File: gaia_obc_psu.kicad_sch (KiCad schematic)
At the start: 49 parts, among them J4 Conn_01x02_Pin, Q1 FS8205A, U10 INA3221, U11 TPS22917DBV, U12 TPS22917DBV, U2 LGS4056H, U3 DW01A, U5 AP2112K-3.3, U8 TPS22917DBV, U9 INA3221

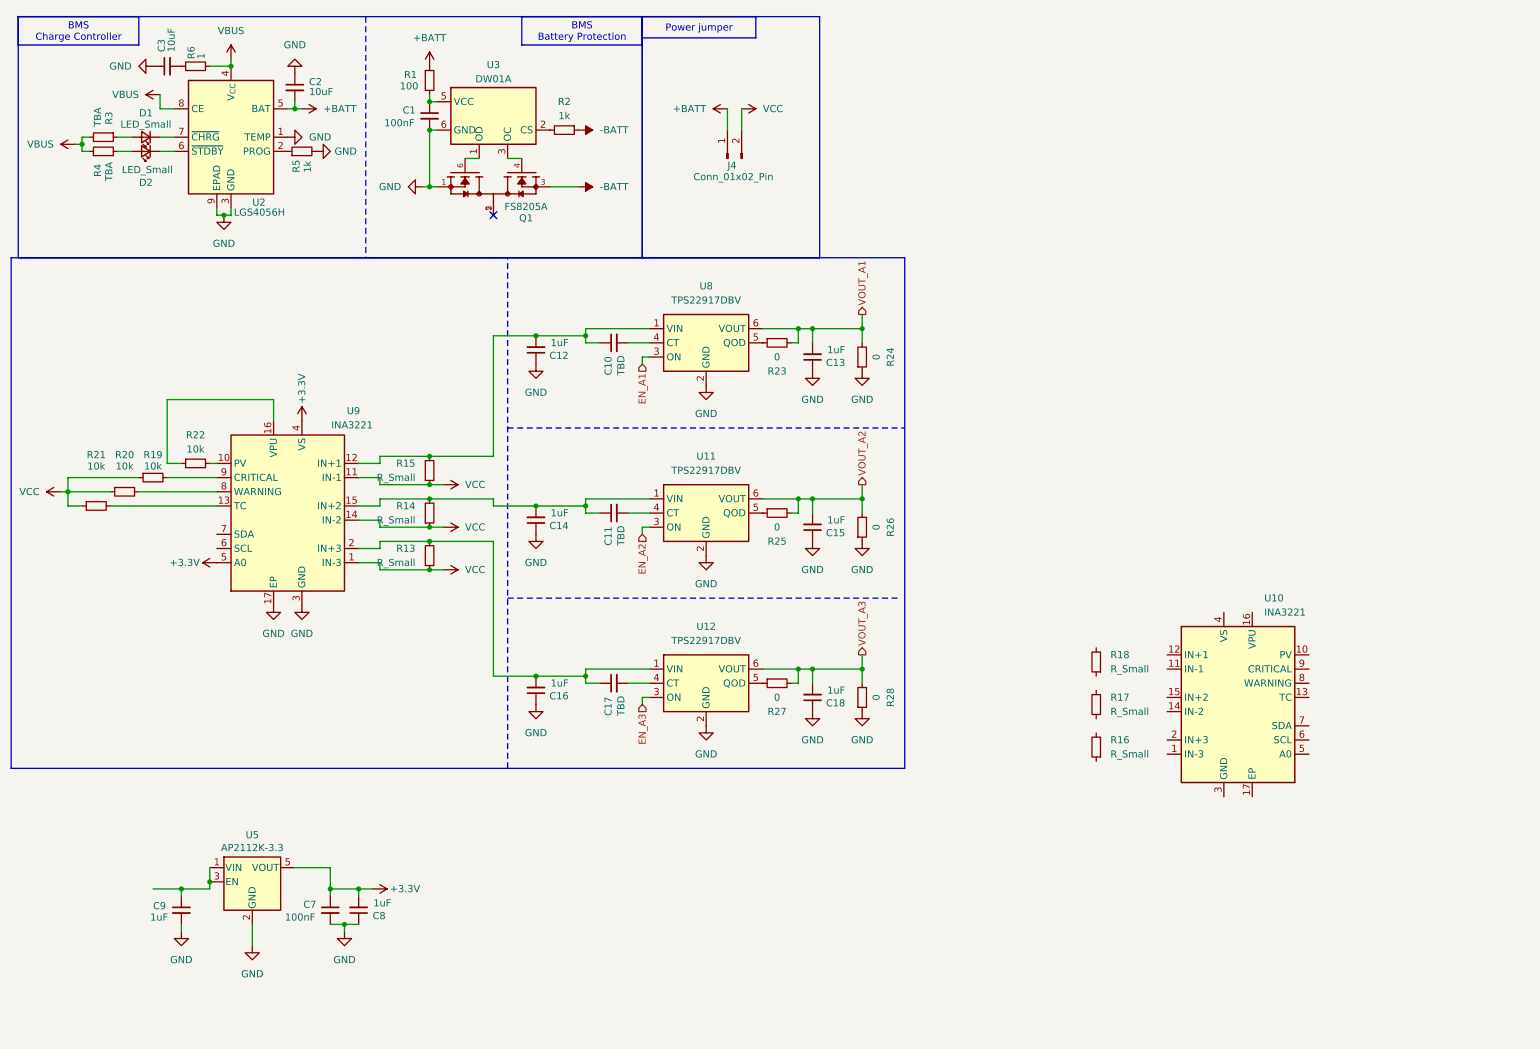
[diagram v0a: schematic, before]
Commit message: finishing psu
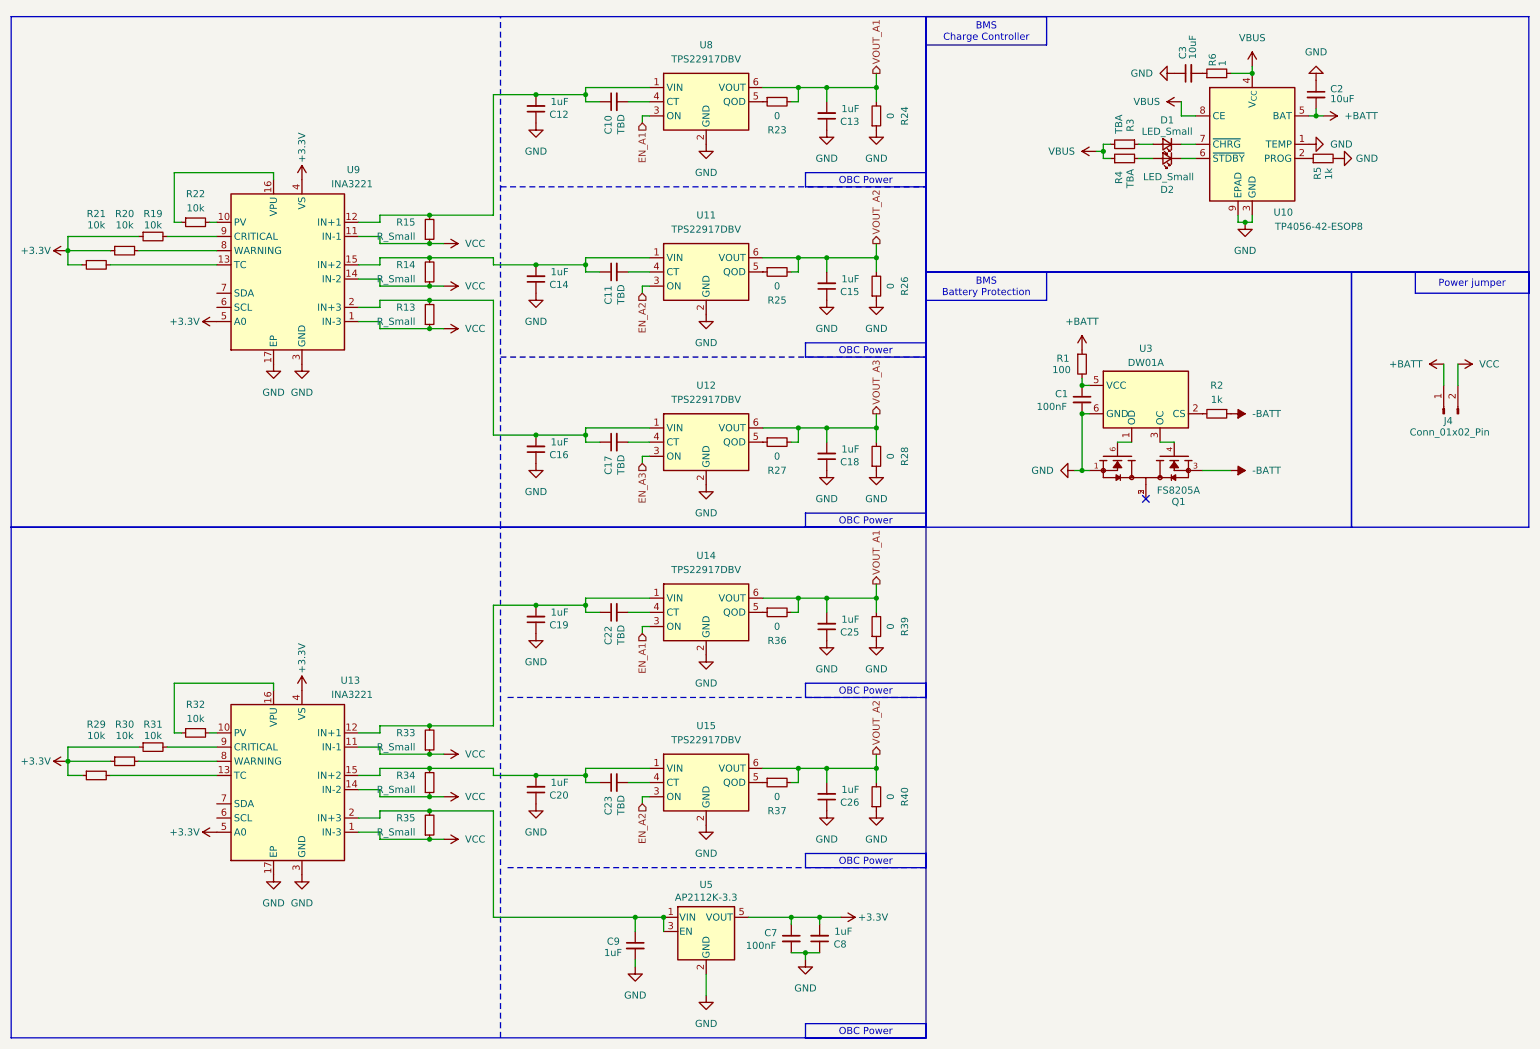
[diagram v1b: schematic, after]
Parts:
- removed R16, R17, R18: R_Small, symbol Device:R_Small
- removed U10: INA3221, Package_DFN_QFN:Texas_RGV0016A_VQFN-16-1EP_4x4mm_P0.65mm_EP2.1x2.1mm, symbol Power_Management:INA3221
- removed U2: LGS4056H, Package_DFN_QFN:DFN-8-1EP_3x3mm_P0.65mm_EP1.7x2.05mm, symbol OnionSAT_Gaia:LGS4056H
- added C19, C20, C25, C26: 1uF, symbol Device:C_Small
- added C22, C23: TBD, symbol Device:C_Small
- added R29, R30, R31, R32: 10k, symbol Device:R_Small
- added R33, R34, R35: R_Small, symbol Device:R_Small
- added R36, R37, R39, R40: 0, symbol Device:R_Small
- added U10: TP4056-42-ESOP8, Package_SO:SOIC-8-1EP_3.9x4.9mm_P1.27mm_EP2.41x3.3mm_ThermalVias, symbol Battery_Management:TP4056-42-ESOP8
- added U13: INA3221, Package_DFN_QFN:Texas_RGV0016A_VQFN-16-1EP_4x4mm_P0.65mm_EP2.1x2.1mm, symbol Power_Management:INA3221
- added U14, U15: TPS22917DBV, Package_TO_SOT_SMD:SOT-23-6, symbol Power_Management:TPS22917DBV
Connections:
- net +3.3V: now also R19.1, R20.1, R21.1, R29.1, R30.1, R31.1, U13.4 (VS), U13.5 (A0)
- net +BATT: now also U10.5 (BAT)
- net EN_A1: now also U14.3 (ON)
- net EN_A2: now also U15.3 (ON)
- net GND: now also C19.1, C20.1, C25.1, C26.1, R39.1, R40.1, U10.1 (TEMP), U10.3 (GND), U10.9 (EPAD), U13.17 (EP), U13.3 (GND), U14.2 (GND), U15.2 (GND)
- net VBUS: now also U10.4 (V_{CC}), U10.8 (CE)
- net VCC: now also R33.1, R34.1, R35.1, U13.1 (IN-3), U13.11 (IN-1), U13.14 (IN-2); no longer R19.1, R20.1, R21.1
- net VOUT_A1: now also C25.2, R36.2, R39.2, U14.6 (VOUT)
- net VOUT_A2: now also C26.2, R37.2, R40.2, U15.6 (VOUT)
- net at R5.1: now also U10.2 (PROG)
- net at D2.1 (K): now also U10.6 (~{STDBY})
- net at D1.1 (K): now also U10.7 (~{CHRG})
- net at C9.1, U5.1 (VIN), U5.3 (EN): now also R35.2, U13.2 (IN+3)
- new net: C19.2, C22.1, R33.2, U13.12 (IN+1), U14.1 (VIN)
- new net: R30.2, U13.8 (WARNING)
- new net: C20.2, C23.1, R34.2, U13.15 (IN+2), U15.1 (VIN)
- new net: C23.2, U15.4 (CT)
- new net: R37.1, U15.5 (QOD)
- new net: C22.2, U14.4 (CT)
- new net: R29.2, U13.13 (TC)
- new net: R32.2, U13.10 (PV)
- new net: R32.1, U13.16 (VPU)
- new net: R31.2, U13.9 (CRITICAL)
- new net: R36.1, U14.5 (QOD)
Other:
- moved on the sheet: C1, C10, C11, C12, C13, C14, C15, C16, C17, C18, C2, C3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
